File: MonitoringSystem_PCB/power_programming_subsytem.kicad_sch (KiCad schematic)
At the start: 17 parts, among them J6 USB_B, Q1 SS8050-G, Q2 SS8050-G, U1 CP2102N-Axx-xQFN28, U6 LM1117MP-3.3

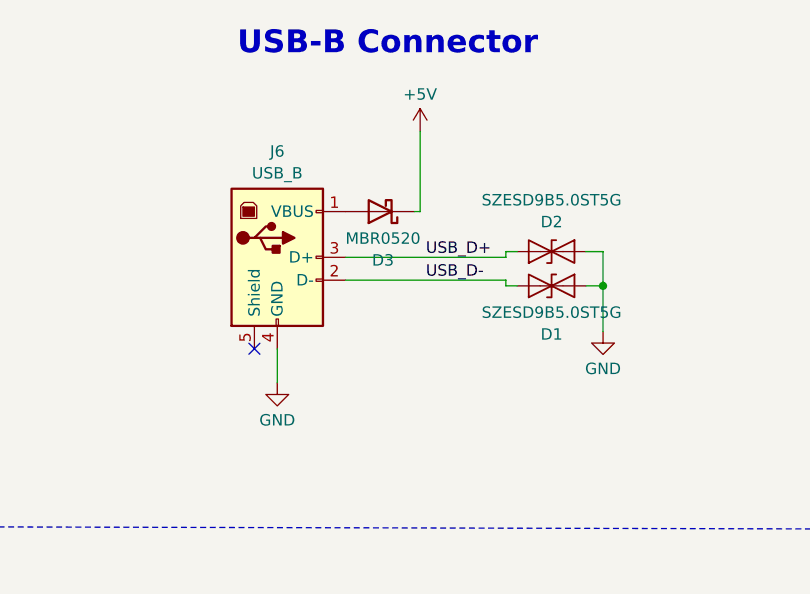
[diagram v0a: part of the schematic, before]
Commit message: finalized pcb, fixed eroors, generated gerber
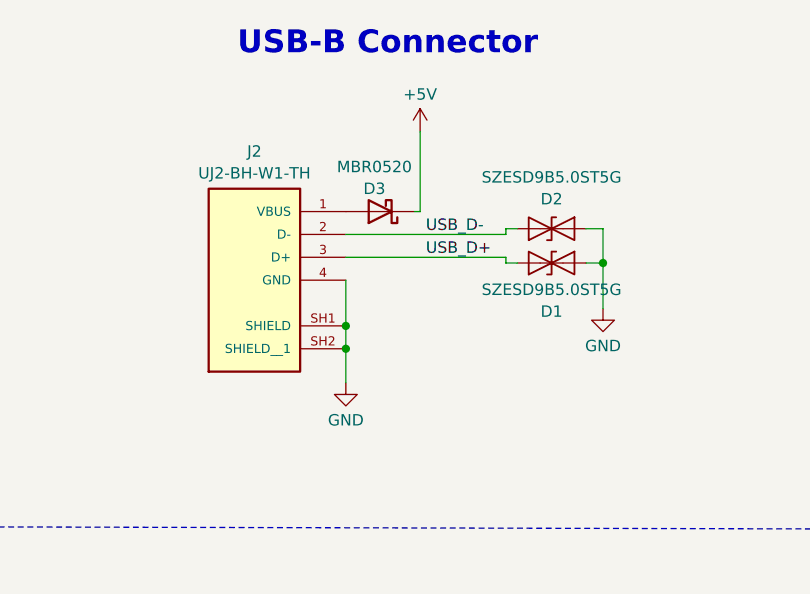
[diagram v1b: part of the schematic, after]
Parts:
- removed J6: USB_B, USB-B:CUI_UJ2-BH-W1-TH, symbol Connector:USB_B
- added J2: UJ2-BH-W1-TH, USB-B:CUI_UJ2-BH-W1-TH, symbol USB-B:UJ2-BH-W1-TH
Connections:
- net GND: now also J2.4 (GND), J2.SH1 (SHIELD), J2.SH2 (SHIELD__1)
- net USB_D+: now also D1.1 (A1), J2.3 (D+); no longer D2.1 (A1)
- net USB_D-: now also D2.1 (A1), J2.2 (D-); no longer D1.1 (A1)
- net at D3.2 (A): now also J2.1 (VBUS)
- no-connect marks 17 -> 16
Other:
- moved on the sheet: D1, D2
